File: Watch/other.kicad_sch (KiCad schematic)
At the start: 18 parts, among them J1 SSD1306, J2 Conn_02x03_Odd_Even, SW2 SW_Push, SW3 SW_Push, SW4 SW_Push, U3 W25Q80EWSNIG, U7 OPT3001DNPRQ1

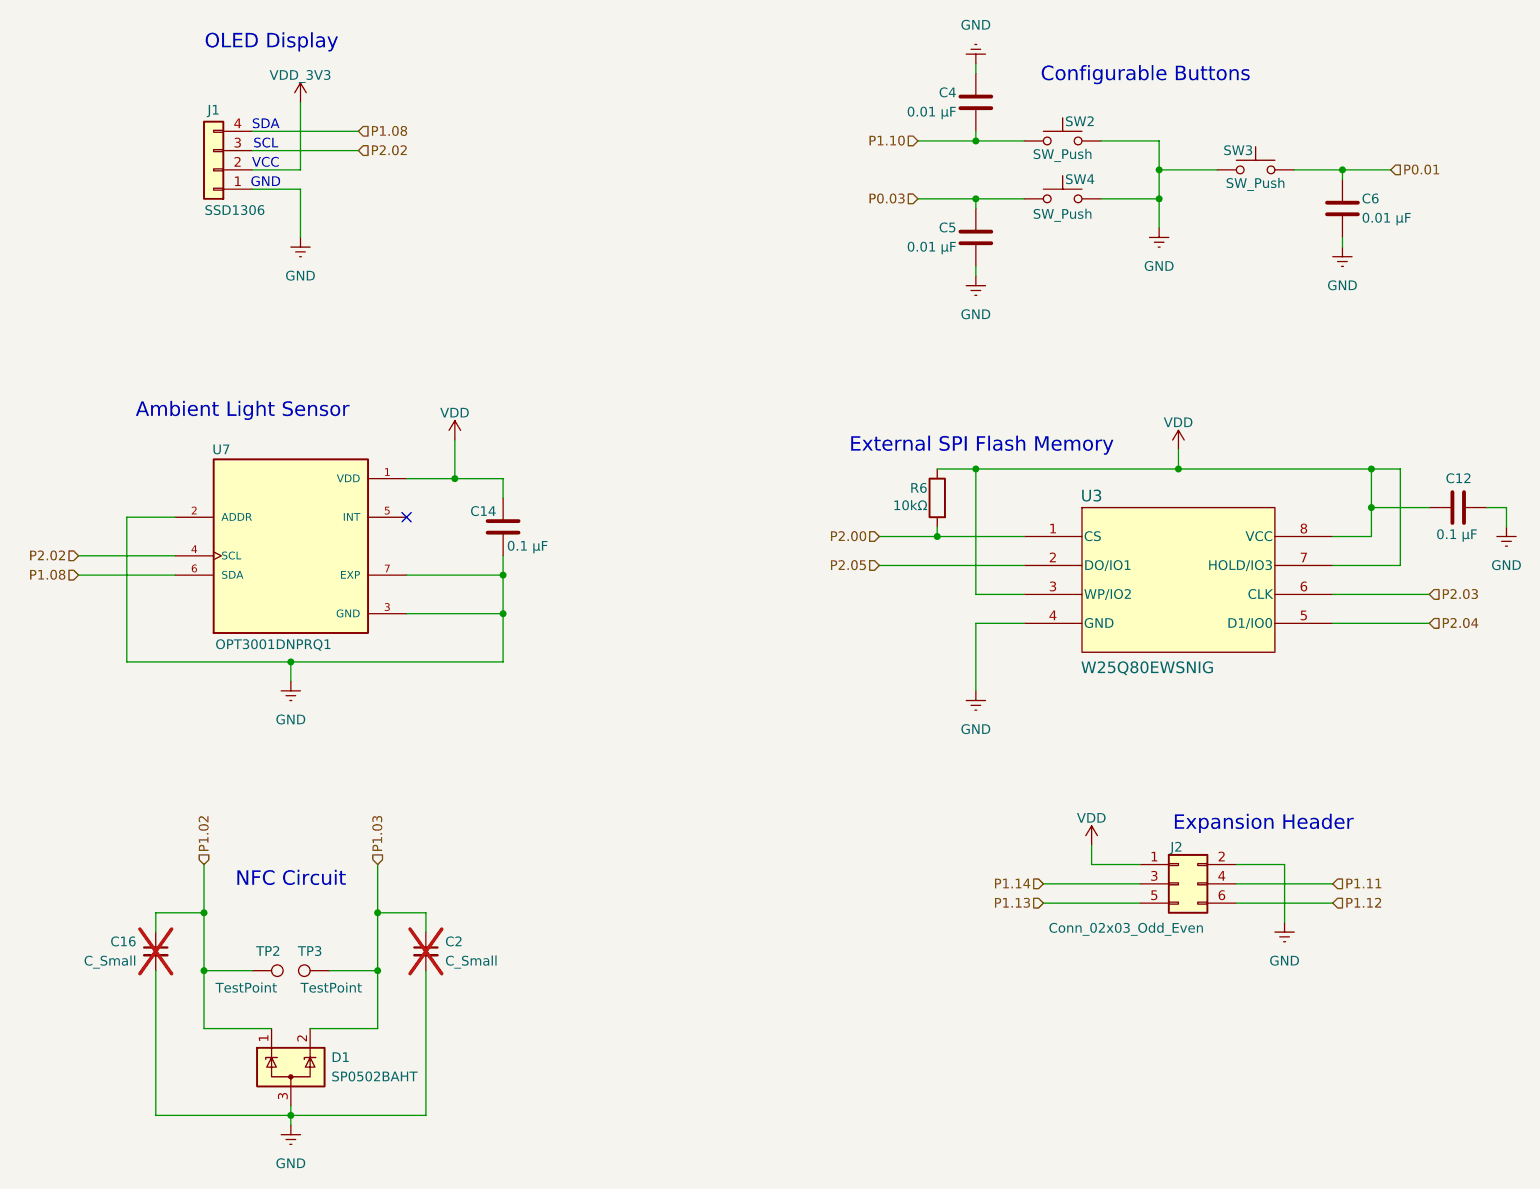
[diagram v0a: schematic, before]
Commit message: Screenshots
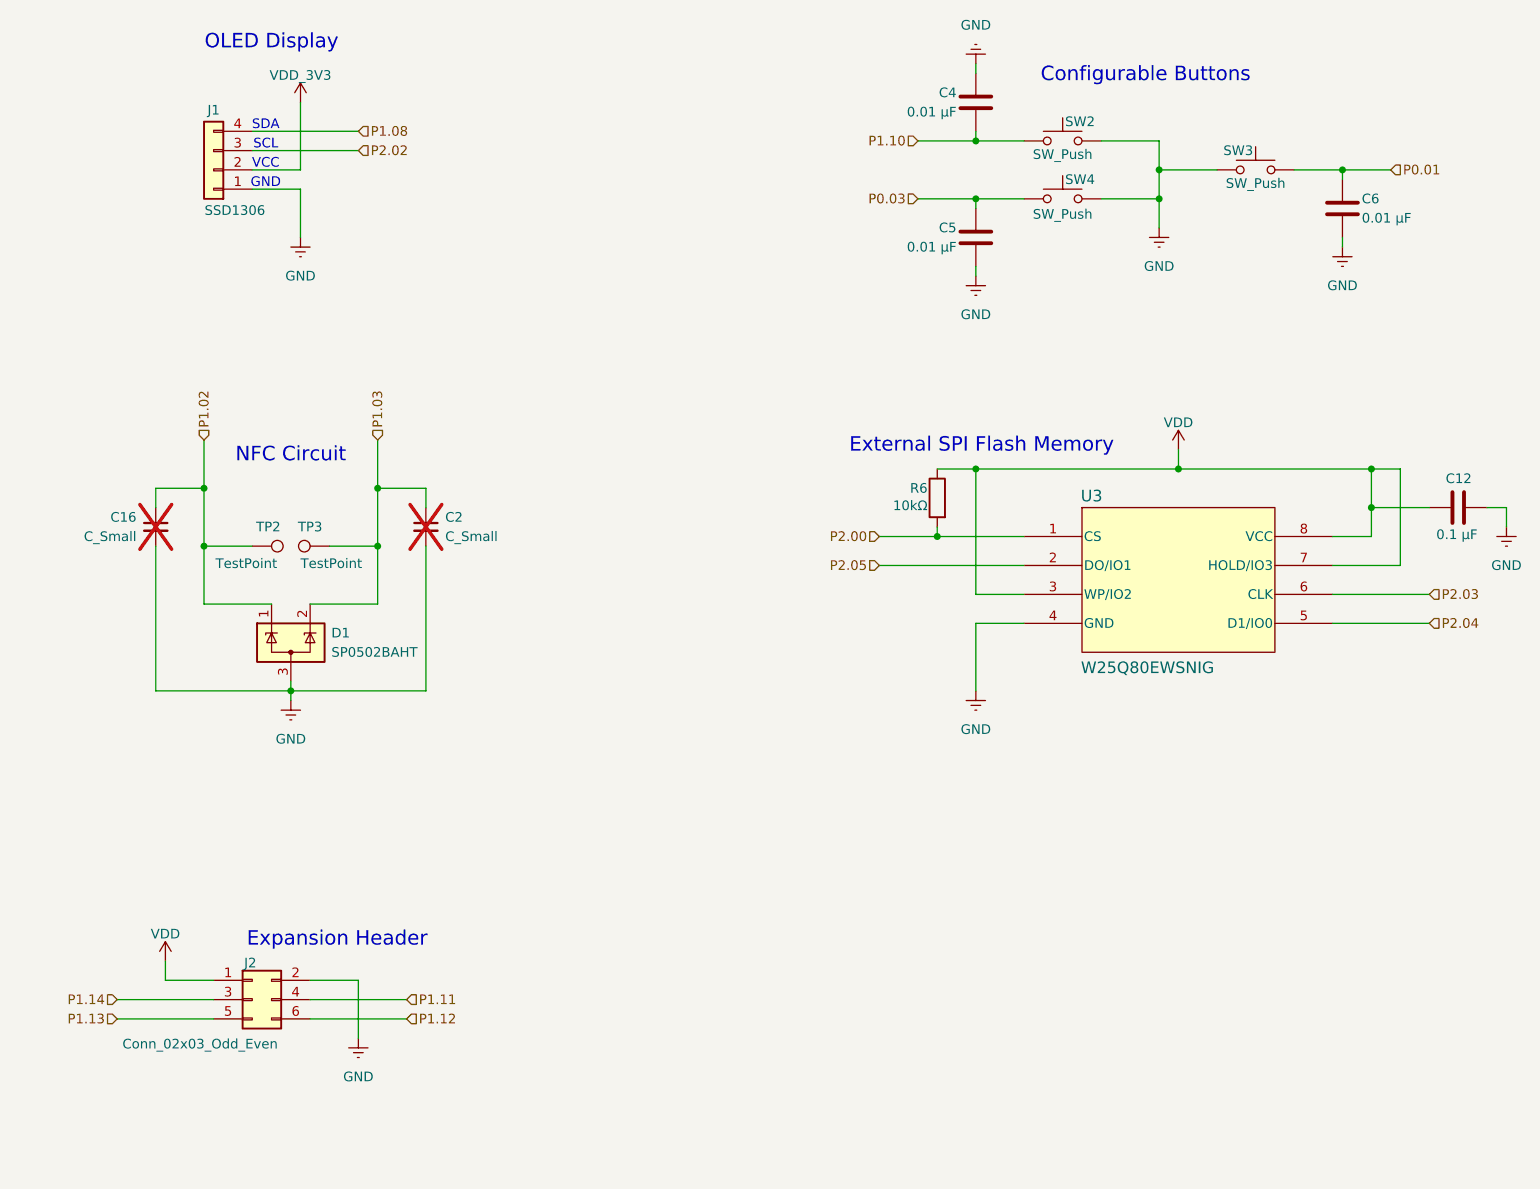
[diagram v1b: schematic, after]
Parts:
- removed C14: 0.1 μF, Capacitor_SMD:C_0402_1005Metric, symbol Device:C
- removed U7: OPT3001DNPRQ1, 1_I_Syst.inc:SON65P200X200X65-7N, symbol I_Syst_inc:OPT3001DNPRQ1
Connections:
- no-connect marks 1 -> 0
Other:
- note removed: "Ambient Light Sensor"
- moved on the sheet: C16, C2, D1, J2, TP2, TP3
